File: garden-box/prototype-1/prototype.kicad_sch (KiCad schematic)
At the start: 33 parts, among them J1 Conn_01x05_Male, J2 Screw_Terminal_01x02, Q1 IRF830, U1 4N35

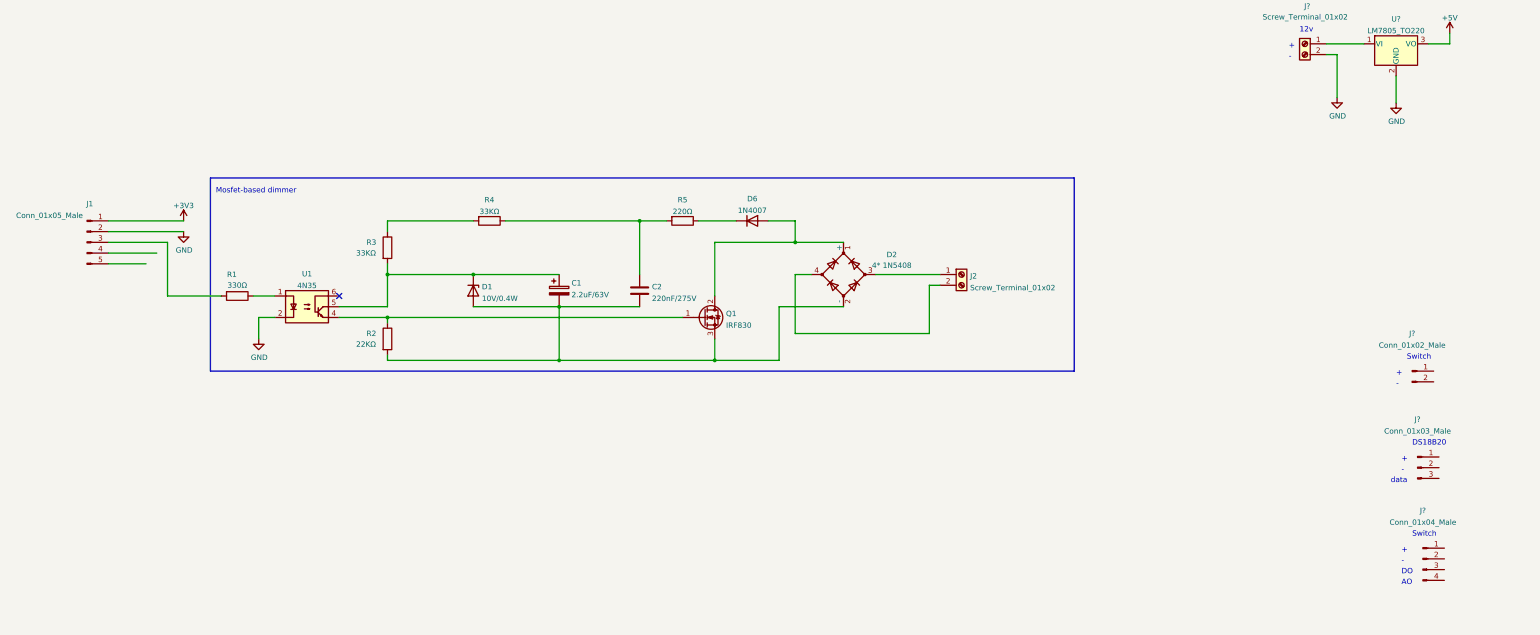
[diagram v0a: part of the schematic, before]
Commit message: wip garden-box schematic
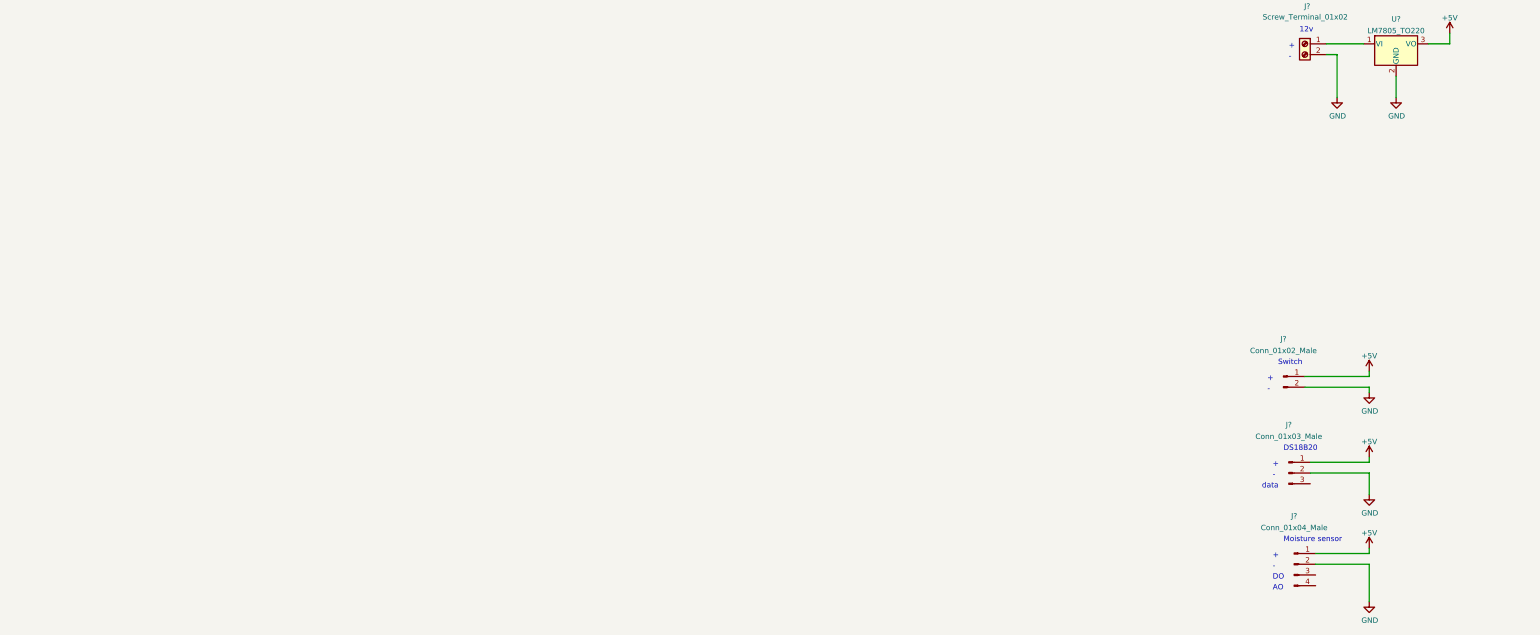
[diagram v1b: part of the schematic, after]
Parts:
- removed C1: 2.2uF/63V, Capacitor_SMD:C_1206_3216Metric, symbol Device:C_Polarized
- removed C2: 220nF/275V, Capacitor_SMD:C_1210_3225Metric, symbol Device:C
- removed D1: 10V/0.4W, Diode_SMD:D_SOD-123, symbol Diode:BZV55B10
- removed D2: 4* 1N5408, Diode_SMD:Diode_Bridge_Diotec_SO-DIL-Slim, symbol Device:D_Bridge_+-AA
- removed D6: 1N4007, Diode_SMD:D_SMA, symbol Diode:1N4007
- removed J1: Conn_01x05_Male, Connector_PinHeader_2.54mm:PinHeader_1x05_P2.54mm_Vertical, symbol Connector:Conn_01x05_Male
- removed J2: Screw_Terminal_01x02, TerminalBlock:TerminalBlock_bornier-2_P5.08mm, symbol Connector:Screw_Terminal_01x02
- removed Q1: IRF830, Package_TO_SOT_SMD:TO-263-3_TabPin2, symbol Transistor_FET:IRF740
- removed R1: 330Ω, Resistor_SMD:R_0603_1608Metric, symbol Device:R
- removed R2: 22KΩ, Resistor_SMD:R_0603_1608Metric, symbol Device:R
- removed R3, R4: 33KΩ, Resistor_SMD:R_0603_1608Metric, symbol Device:R
- removed R5: 220Ω, Resistor_SMD:R_0603_1608Metric, symbol Device:R
- removed U1: 4N35, Package_DIP:SMDIP-6_W7.62mm, symbol Isolator:4N35
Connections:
- net +5V: now also J?.1 (Pin_1), J?.1 (Pin_1), J?.1 (Pin_1)
- net GND: now also J?.2 (Pin_2), J?.2 (Pin_2), J?.2 (Pin_2)
- no-connect marks 1 -> 0
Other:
- note added: "Moisture sensor"
- note removed: "Mosfet-based dimmer"
- moved on the sheet: J?
